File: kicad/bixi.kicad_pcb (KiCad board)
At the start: 2 copper layers, 105 x 107.5 mm, 38 parts, among them CON1 BARREL_JACK, J1 RJ45, J2 RJ45, J3 RJ45, J4 RJ45, J5 RJ45, J6 RJ45, J7 RJ45, J8 RJ45, U1 Teensy3.6, U2 SP3485CN, U3 SP3485CN, U4 SP3485CN, U5 SP3485CN, U6 SP3485CN, U7 SP3485CN, U8 SP3485CN, U9 SP3485CN

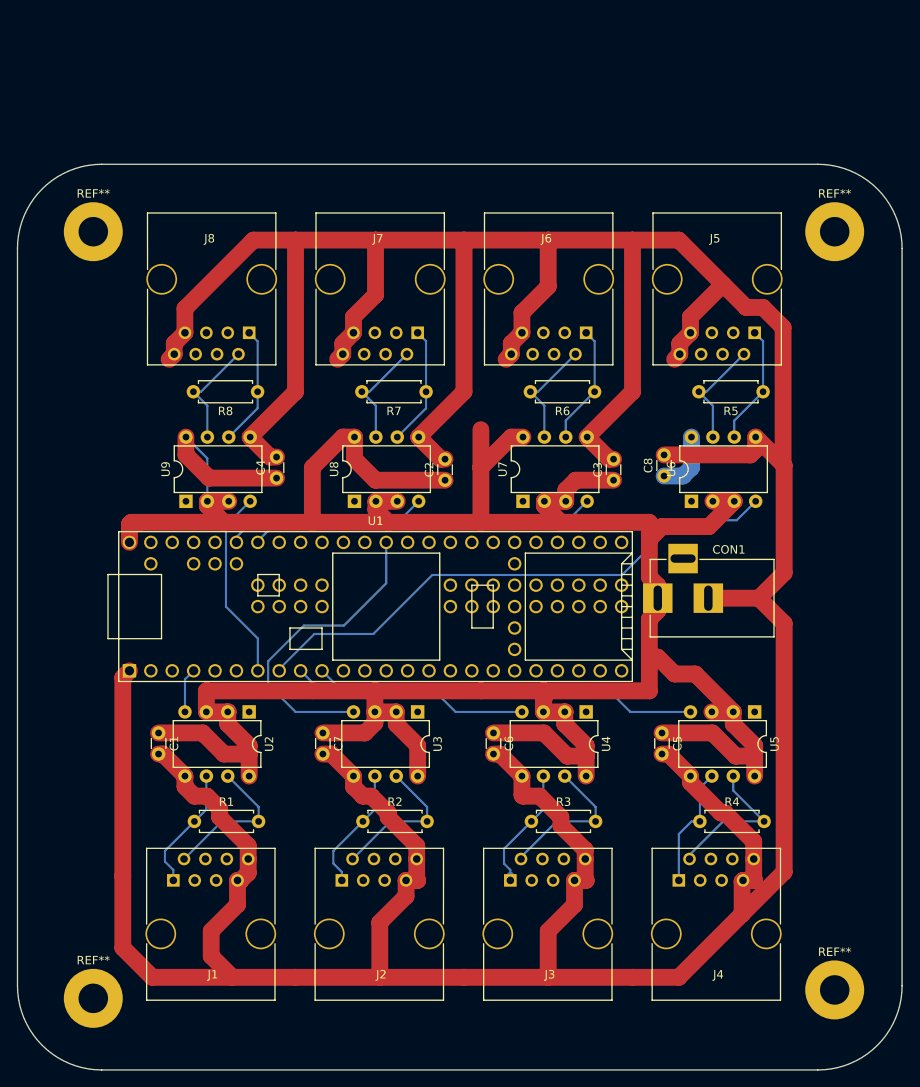
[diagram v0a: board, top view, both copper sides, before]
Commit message: controller and receiver boards almost done for v1
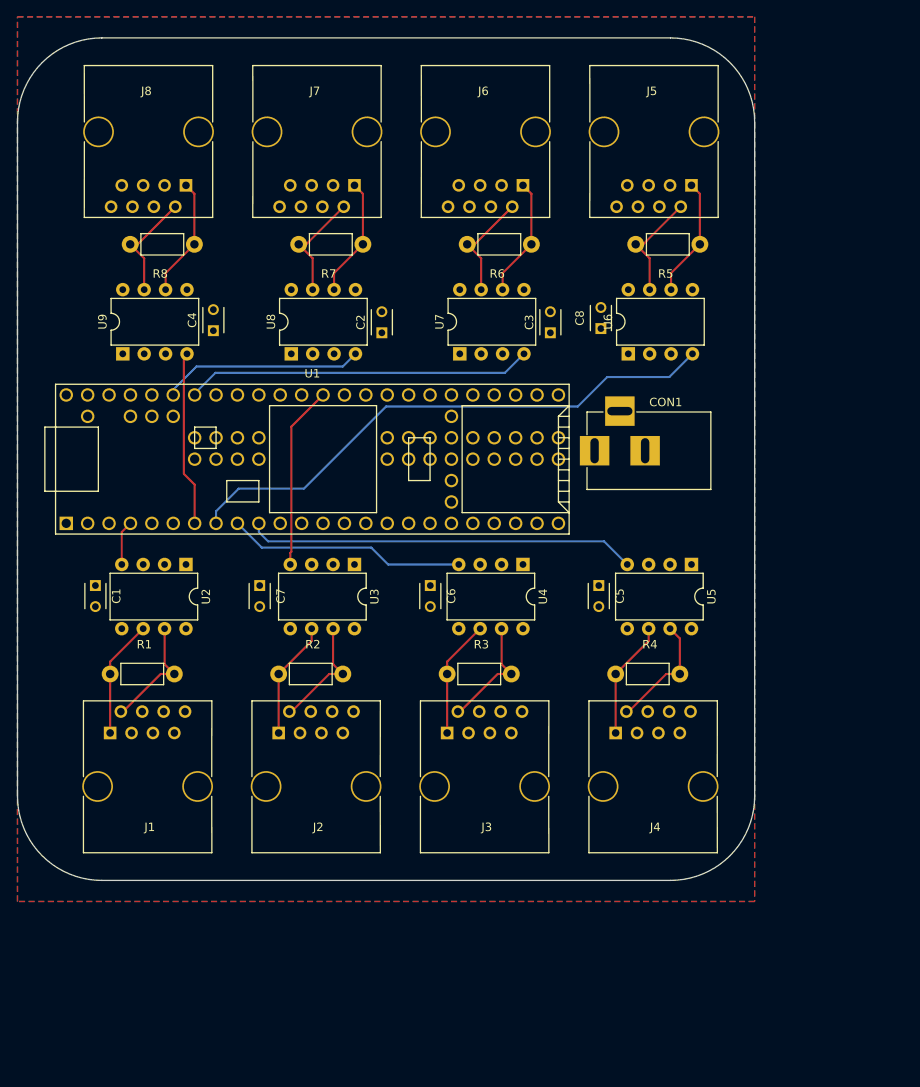
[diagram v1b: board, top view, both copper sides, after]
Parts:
- removed REF** (x4): MountingHole_3.5mm_Pad, Mounting_Holes:MountingHole_3.5mm_Pad
- C1, C2, C3, C4, C5, C6, C7, C8: footprint Capacitors_THT:C_Disc_D3.0mm_W1.6mm_P2.50mm -> Capacitors_THT:C_Disc_D3_P2.5
- R1, R2, R3, R4, R5, R6, R7, R8: footprint Resistors_THT:R_Axial_DIN0207_L6.3mm_D2.5mm_P7.62mm_Horizontal -> Resistors_THT:Resistor_Horizontal_RM7mm
- moved R1 20.2 mm to (106.0, 120.5)
- moved R2 20.2 mm to (126.0, 120.5)
- moved R3 20.2 mm to (146.0, 120.5)
- moved R4 20.2 mm to (166.0, 120.5)
- moved C1 19.0 mm to (104.2, 110.0)
- moved C2 19.0 mm to (138.2, 80.0)
- moved C3 19.0 mm to (158.2, 80.0)
- moved C4 19.0 mm to (118.2, 79.8)
- moved C5 19.0 mm to (164.0, 110.0)
- moved C6 19.0 mm to (144.0, 110.0)
- moved C7 19.0 mm to (123.8, 110.0)
- moved C8 19.0 mm to (164.2, 79.5)
- moved CON1 19.0 mm to (163.5, 94.0)
- moved J1 19.0 mm to (106.0, 127.5)
- moved J2 19.0 mm to (126.0, 127.5)
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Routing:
- net GND: track 558.3 -> 0.00 mm
- net VCC: track 366.8 -> 0.00 mm
- net /WS_2: track 36.9 -> 21.7 mm
- net Net-(J4-Pad2): track 17.9 -> 14.1 mm
- net Net-(J3-Pad2): track 17.7 -> 14.1 mm
- net Net-(J1-Pad2): track 17.6 -> 14.1 mm
- net Net-(J2-Pad2): track 17.6 -> 14.1 mm
- net /WS_8: track 22.9 -> 20.8 mm
- net Net-(J3-Pad1): track 15.1 -> 14.0 mm
- net Net-(J2-Pad1): track 14.8 -> 14.0 mm
- net Net-(J1-Pad1): track 14.8 -> 14.0 mm
- net /WS_5: track 65.0 -> 65.7 mm
- net /WS_4: track 45.8 -> 46.4 mm
- net Net-(J4-Pad1): track 14.6 -> 14.0 mm
- added copper zone on B.Cu, net GND
- added copper zone on F.Cu, net VCC
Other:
- board size 105 x 107.5 mm -> 87.5 x 100 mm
- net class Default: trace_width 2 -> 0.25
